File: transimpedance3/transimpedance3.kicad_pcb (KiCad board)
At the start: 2 copper layers, 28.7 x 15.5 mm, 16 parts, among them P1 CONN_01X04, P2 CONN_01X04, P3 10k, U1 DUALOPAMP

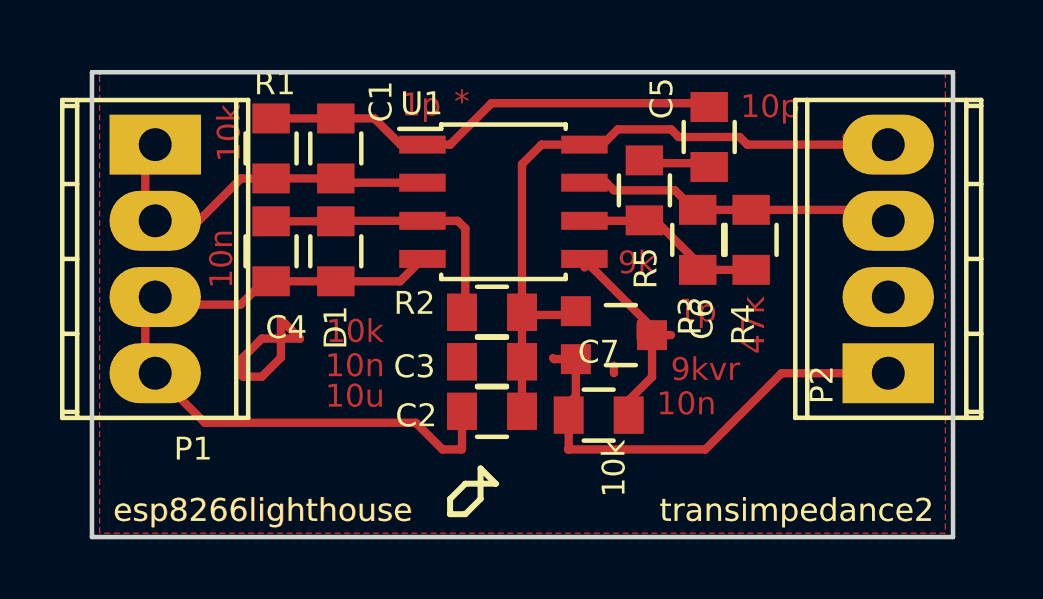
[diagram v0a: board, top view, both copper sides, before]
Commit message: Update all designs with newest to fab.
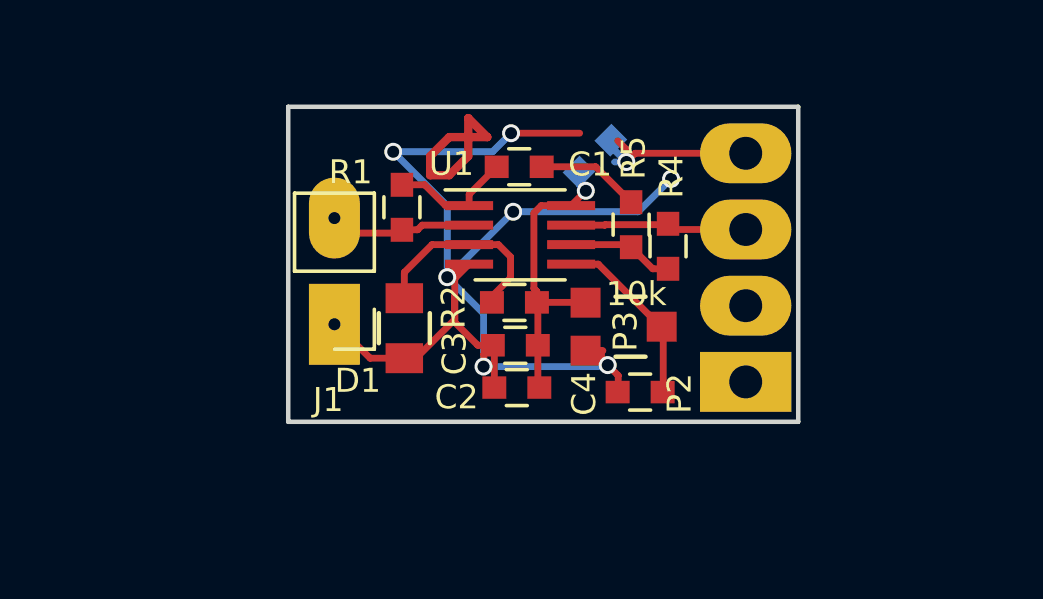
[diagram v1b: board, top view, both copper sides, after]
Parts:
- removed C5: 10p, C_0805
- removed C6: 1p, C_0805
- removed C7: 10n, C_0805
- removed P1: CONN_01X04, TerminalBlock_Pheonix_MPT-2.54mm_4pol
- added J1: PHOTO, Pin_Header_Straight_1x02_Pitch2.54mm, F.Cu at (45.4, 39.5)
- added R3: J, C_0603, B.Cu at (54.1, 34.4)
- C1: value .1p -> 36pF; footprint C_0805 -> C_0603
- C2, C3, C4, R1, R2, R4: footprint C_0805 -> C_0603
- P2: value CONN_01X04 -> SYS
- R5: value 10k -> 4.7k; footprint C_0805 -> C_0603
- U1: value DUALOPAMP -> TSV992; footprint SOIC-8_3.9x4.9mm_Pitch1.27mm -> Housings_SSOP:SSOP-8_2.95x2.8mm_Pitch0.65mm
- moved C4 13.2 mm to (55.6, 42.3), turned to 0 degrees
- moved C1 6.14 mm to (51.6, 34.8), turned to 180 degrees
- moved R1 4.78 mm to (47.7, 36.1)
- moved P2 4.76 mm to (59.1, 41.9)
- moved D1 3.43 mm to (47.8, 40.2)
- moved R4 2.78 mm to (56.5, 37.4)
- moved U1 1.24 mm to (51.6, 37.0)
- moved R5 1.23 mm to (55.3, 36.7)
- moved C2 1.14 mm to (51.5, 42.1)
- moved C3 0.95 mm to (51.5, 40.7)
- moved R2 0.82 mm to (51.4, 39.3)
- moved P3 0.43 mm to (53.8, 40.1)
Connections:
- C4 pad 1: VG1 -> GND
- C4 pad 2: GND -> Net-(C4-Pad2)
- P2 pad 4: +3V3 -> Net-(P2-Pad4)
- P3 pad 2: Net-(C7-Pad2) -> Net-(C4-Pad2)
- R1 pad 1: Net-(C1-Pad1) -> Net-(C1-Pad2)
- R1 pad 2: Net-(C1-Pad2) -> Net-(J1-Pad2)
- R5 pad 2: Net-(C5-Pad1) -> Net-(C1-Pad1)
- U1 pad 1: Net-(C1-Pad1) -> Net-(C1-Pad2)
- U1 pad 2: Net-(C1-Pad2) -> Net-(J1-Pad2)
- U1 pad 5: Net-(C7-Pad2) -> Net-(C4-Pad2)
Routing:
- net +3V3: track 23.2 -> 10.3 mm, vias 0 -> 1
- net Net-(C1-Pad1): track 15.5 -> 3.47 mm
- net Net-(C7-Pad2): track 8.39 -> 0.00 mm
- net Net-(C1-Pad2): track 12.5 -> 4.20 mm
- net Net-(P2-Pad4): track 0.00 -> 6.26 mm, vias 0 -> 1
- net Net-(C4-Pad2): track 0.00 -> 5.80 mm
- net Net-(P2-Pad3): track 10.6 -> 5.92 mm
- net Net-(J1-Pad2): track 0.00 -> 4.60 mm
- net Net-(R4-Pad2): track 7.05 -> 3.56 mm
- net VG1: track 9.43 -> 6.73 mm
- net GND: track 41.3 -> 43.8 mm, vias 0 -> 7
- net Net-(C5-Pad1): track 2.20 -> 0.00 mm
- added copper zone on B.Cu, net GND
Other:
- board size 28.7 x 15.5 mm -> 17 x 10.5 mm
- net class Default: clearance 0.2794 -> 0.2032; trace_width 0.2794 -> 0.2286
- rule pad_to_mask_clearance: 0.2 -> 0.1016
- rule trace_clearance: 0.2794 -> 0.2032
- board text added: "+"
- board text added: "-"
- board text added: "transimpedance3 Rev - C. Lohr, 2017"
- board text removed: "*"
- board text removed: "10k"
- board text removed: "10n"
- board text removed: "10p"
- board text removed: "10u"
- board text removed: "1p"
- board text removed: "47k"
- board text removed: "9k"
- board text removed: "9kvr"
- board text removed: "transimpedance2"
